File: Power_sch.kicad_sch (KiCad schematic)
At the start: 13 parts, among them J1 USB4105-GF-A, J2 USB4105-GF-A, U1 LD39200PU33R, U2 TPD2EUSB30ADRTR

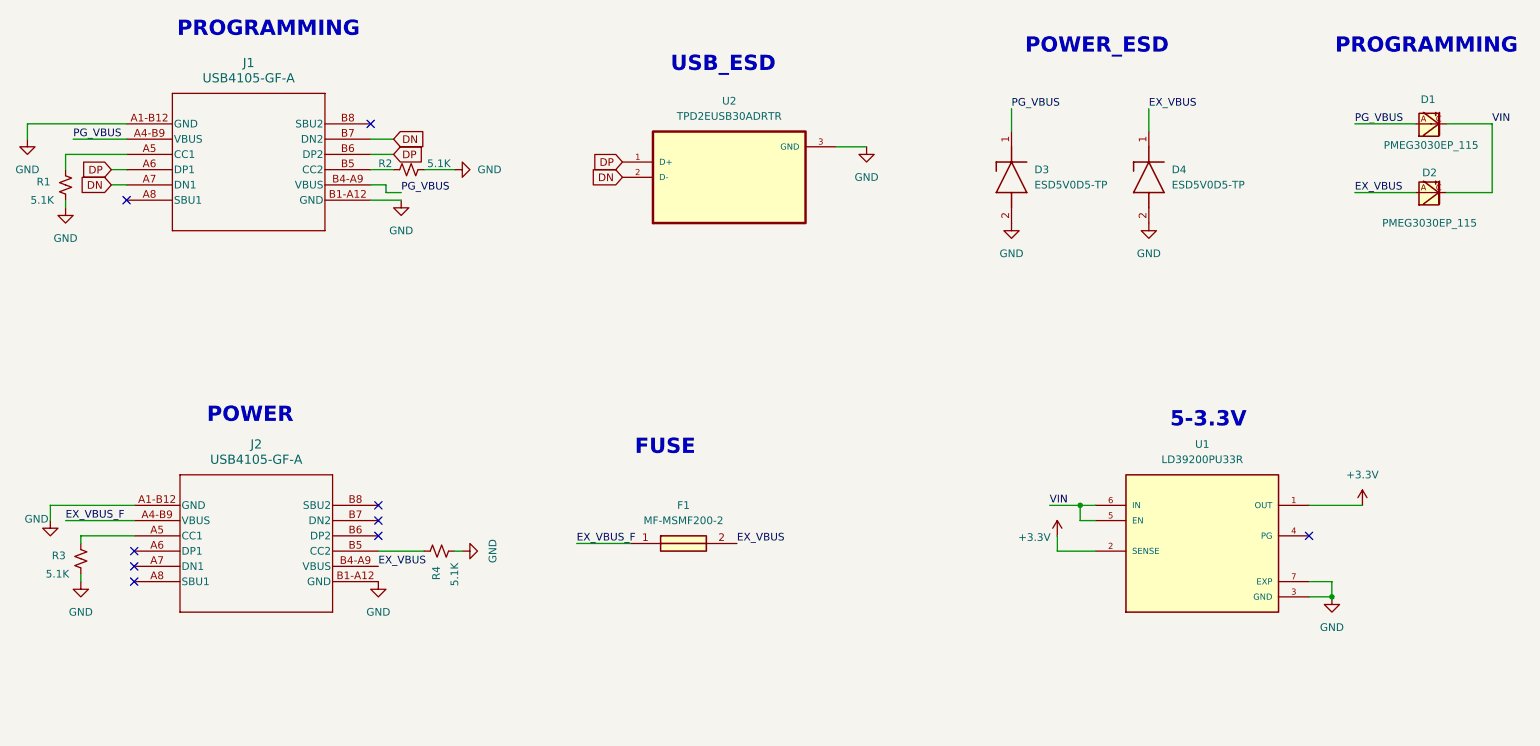
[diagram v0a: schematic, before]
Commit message: Updata the USB Hub Sheet
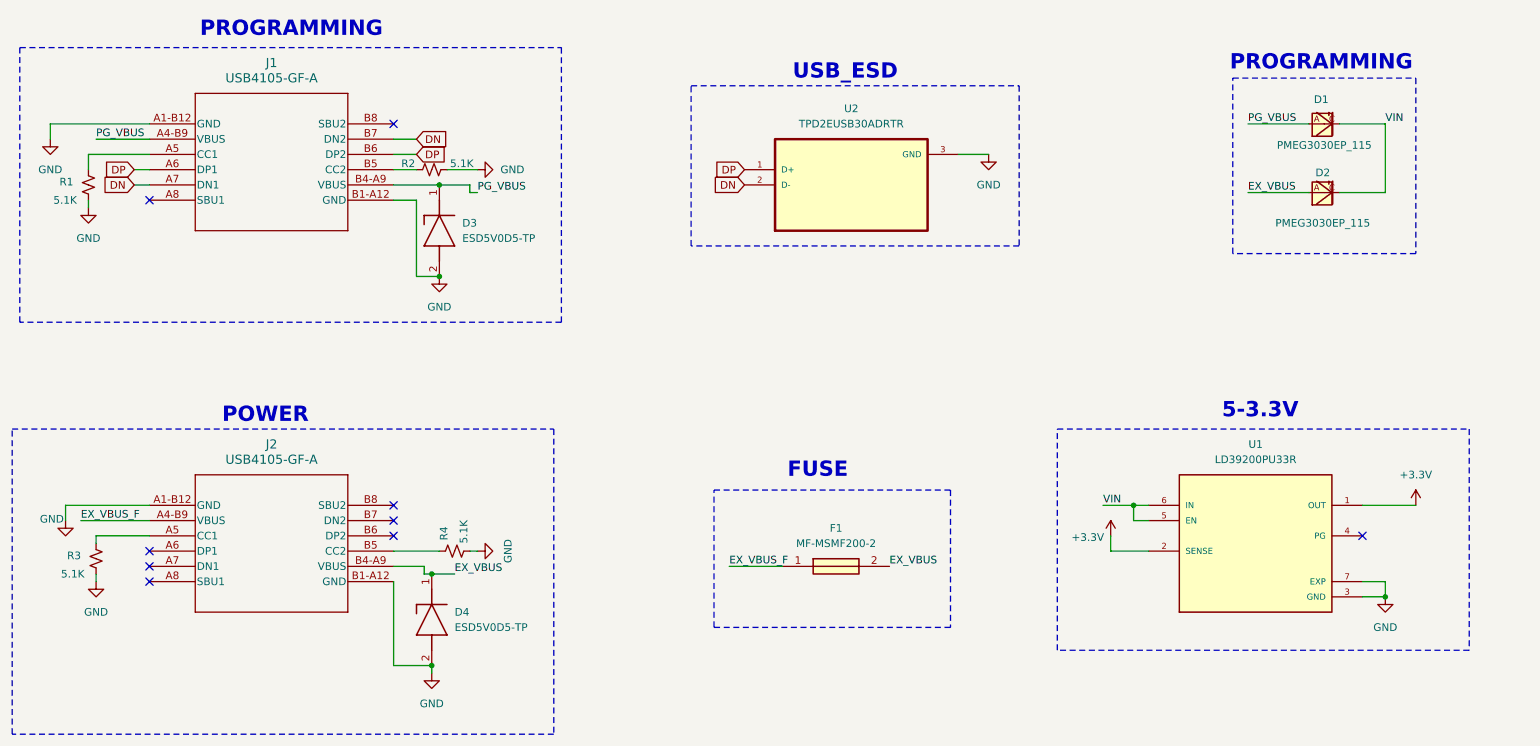
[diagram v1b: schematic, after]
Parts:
- R1: footprint (none) -> Resistor_SMD:R_0402_1005Metric
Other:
- note removed: "POWER_ESD"
- moved on the sheet: D3, D4, F1, J1, J2, R1, R2, R3, R4, U1, U2
